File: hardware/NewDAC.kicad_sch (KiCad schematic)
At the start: 63 parts, among them J1 PJ-322, U1 PCM1795, U14 OPA1656, U15 OPA1656, U6 LM4562, U7 LM4562

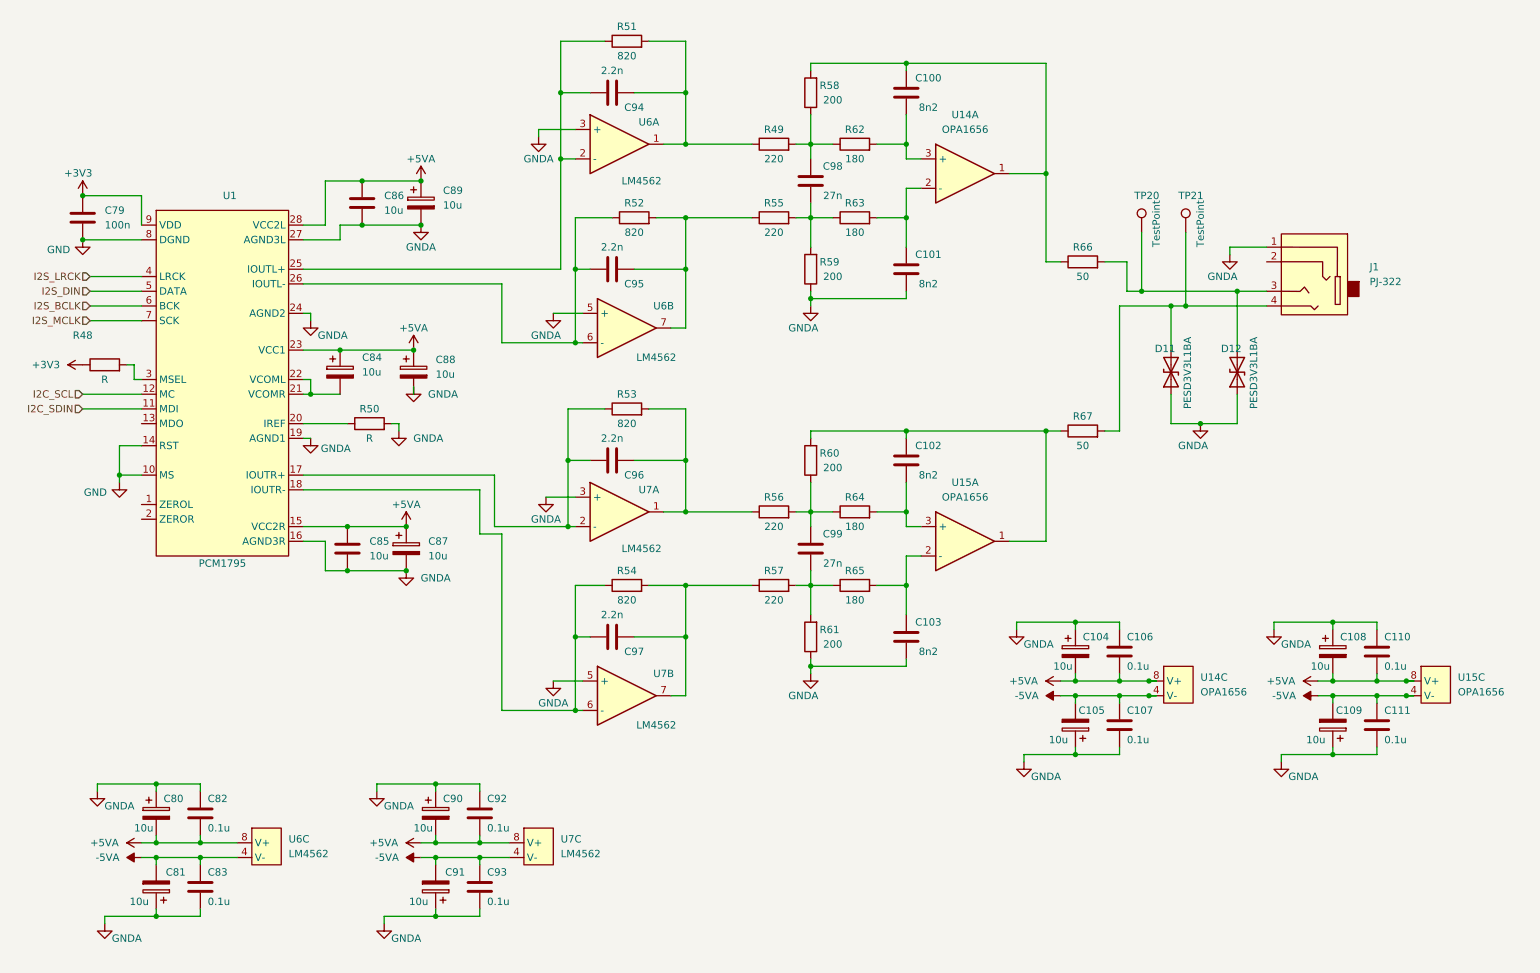
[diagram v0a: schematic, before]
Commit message: some chnages
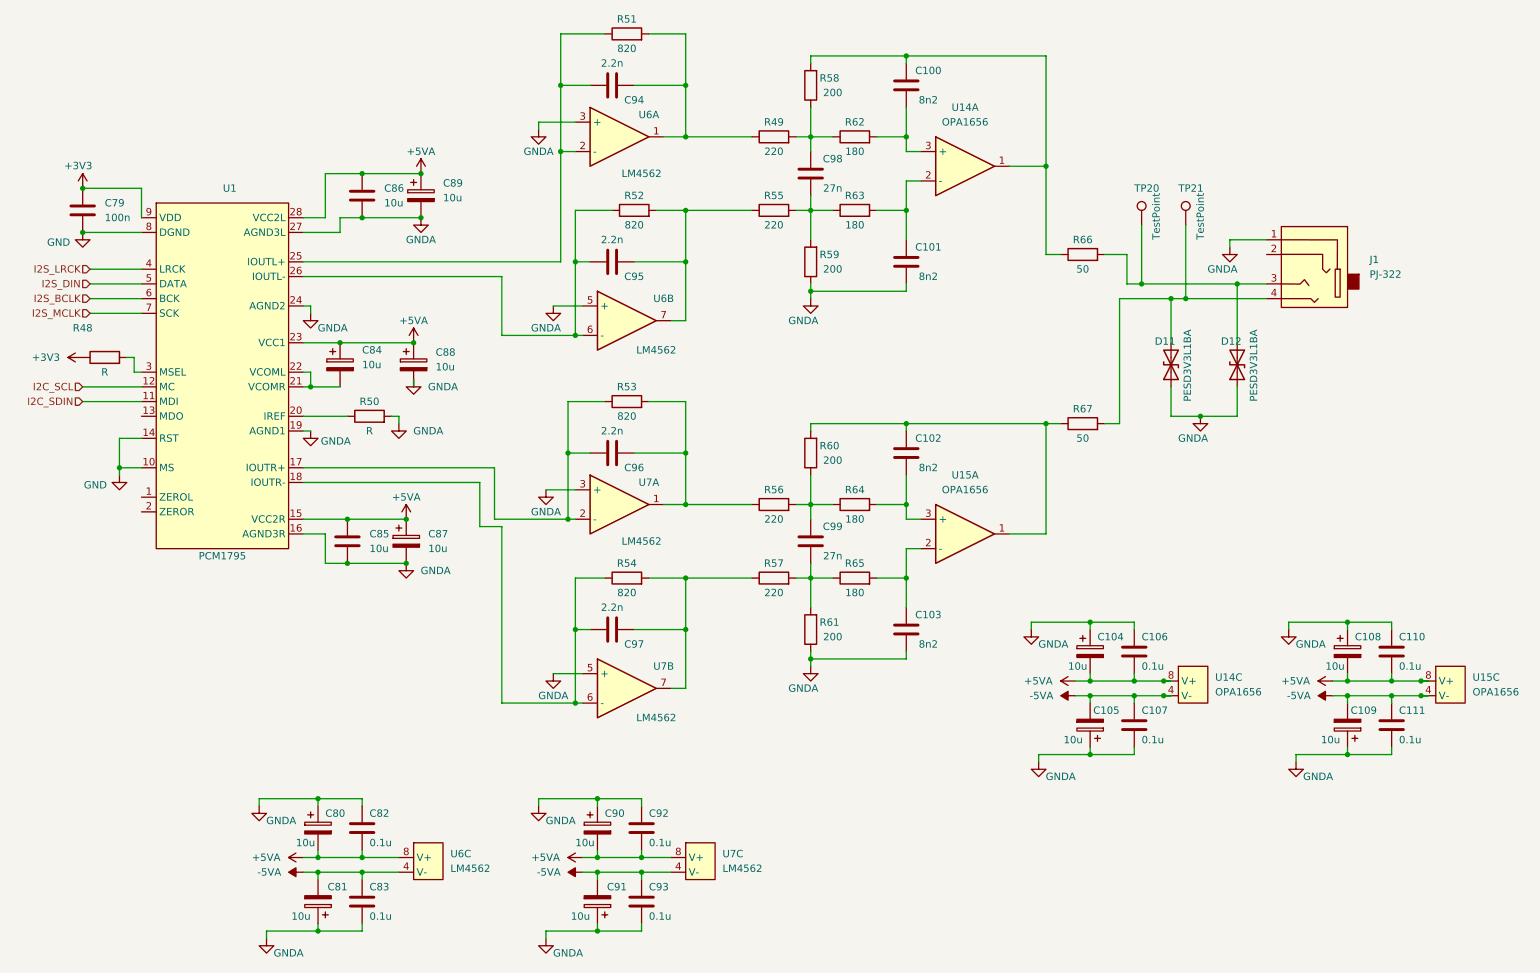
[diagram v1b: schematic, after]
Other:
- moved on the sheet: C100, C101, C102, C103, C104, C105, C106, C107, C108, C109, C110, C111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
